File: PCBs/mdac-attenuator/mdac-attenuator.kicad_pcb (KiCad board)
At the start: 2 copper layers, 45.7 x 52.1 mm, 34 parts, among them J1 Conn_01x06_Male, J2 Conn_01x06_Male, U1 AD8620, U2 DAC8812ICPWG4

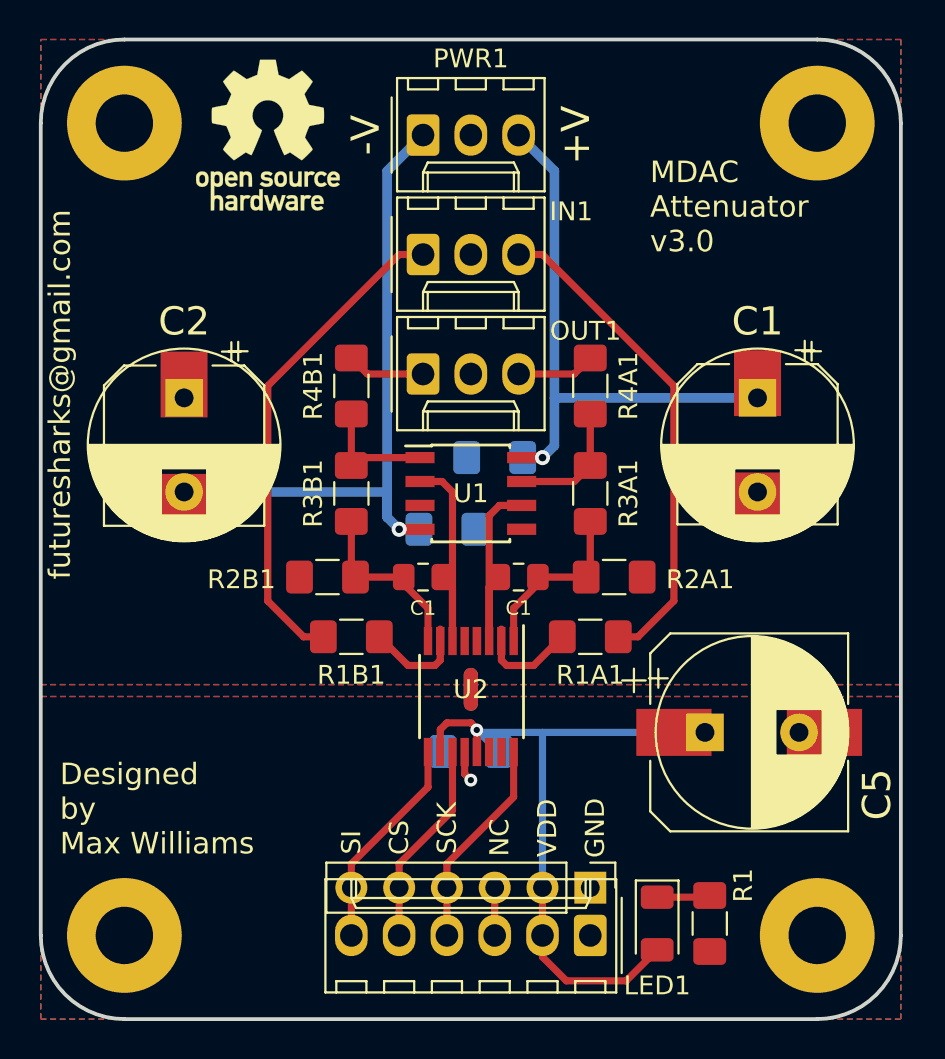
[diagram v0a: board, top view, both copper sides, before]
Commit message: Misc updates to 3 PCBs
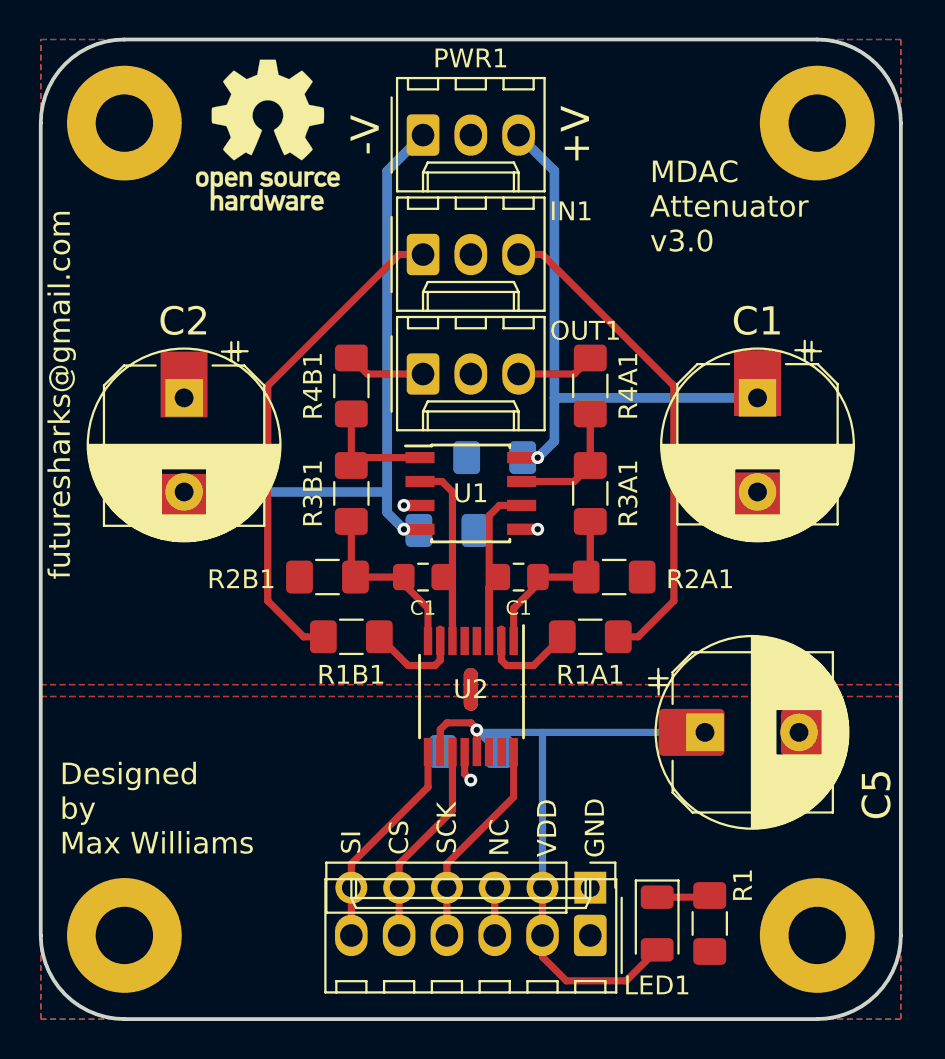
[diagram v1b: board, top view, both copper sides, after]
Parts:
- C5_SMD1: footprint Capacitor_SMD:CP_Elec_10x10 -> Capacitor_SMD:CP_Elec_8x10
- moved C5_SMD1 0.19 mm to (161.0, 110.5)
- moved C4 0.06 mm to (144.8, 99.8)
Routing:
- net -15V: track 37.1 -> 35.5 mm
- net +15V: track 31.2 -> 29.9 mm
- net GNDA: vias 1 -> 3
